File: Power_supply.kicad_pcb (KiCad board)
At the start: 2 copper layers, 160 x 40 mm, 51 parts, among them J1 Transformers, J20 HV_Transformer, J21 LV_Transformer, J22 220V, J23 Transformers, J24 Thyratrone, J25 Anodes_enable, J26 Conn_01x04, J27 Conn_01x04, J28 Conn_01x04, K2 SANYOU_SRD_Form_C, Q10 MPSA42, Q11 STP4NK60ZFP(MJE13003), Q12 2N3904, U4 SG2P

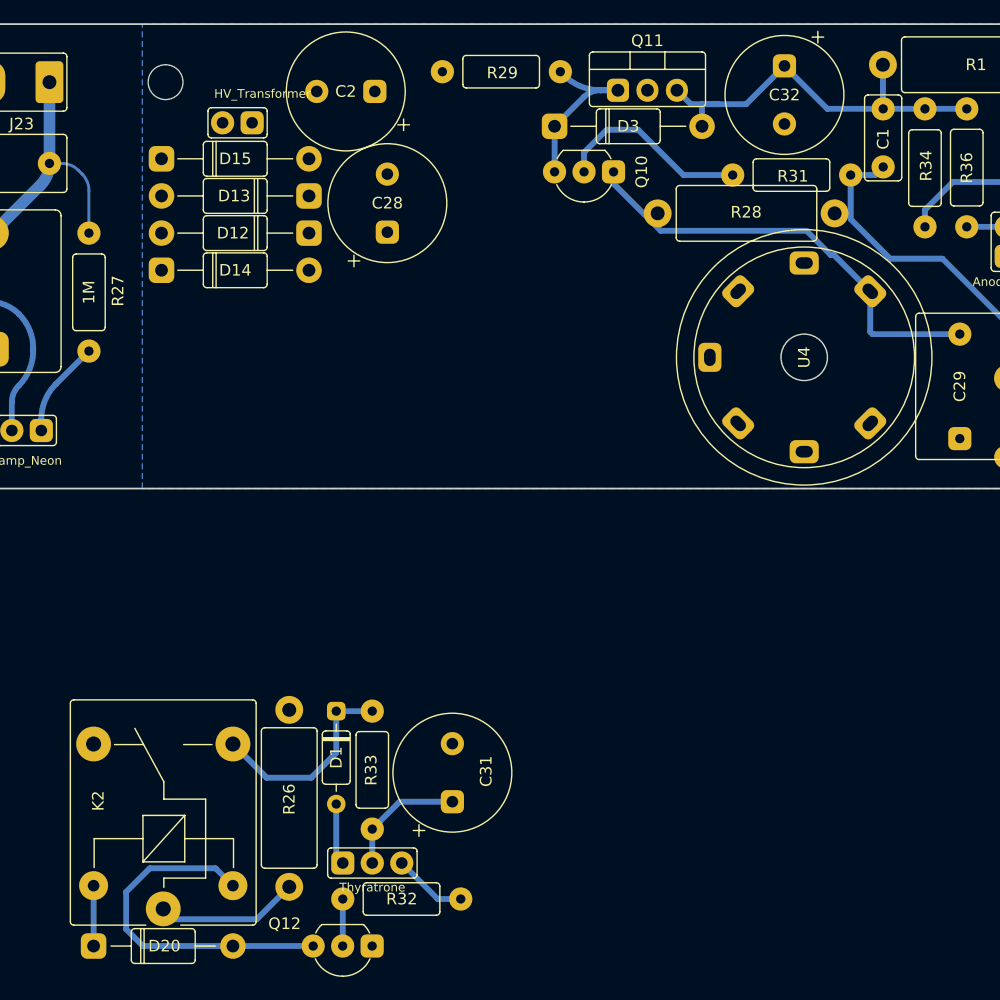
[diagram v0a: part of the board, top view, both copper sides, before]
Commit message: Working on power supply PCB
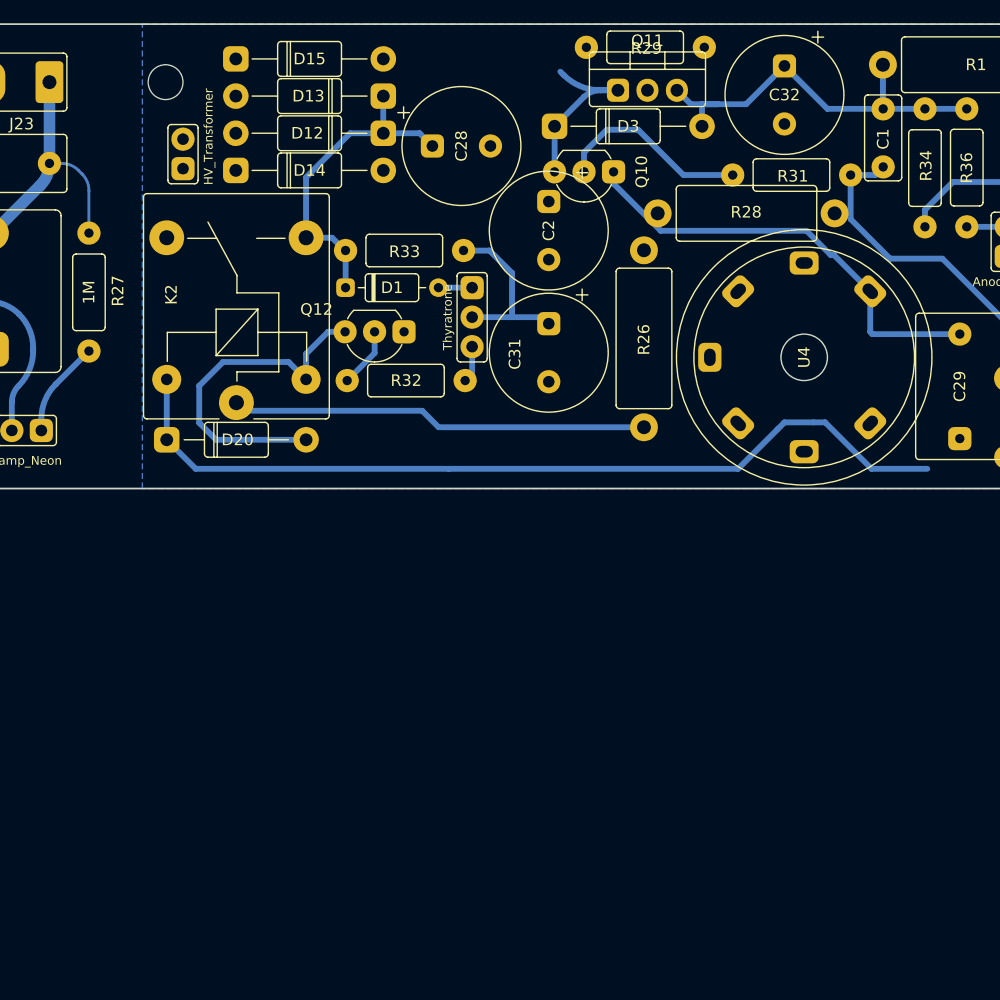
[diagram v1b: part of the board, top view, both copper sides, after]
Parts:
- moved Q12 53.0 mm to (80.0, 116.5)
- moved J24 50.8 mm to (88.4, 112.7), turned to 0 degrees
- moved R33 50.4 mm to (87.7, 109.5), turned to 180 degrees
- moved R26 50.0 mm to (103.2, 124.7)
- moved R32 44.7 mm to (87.8, 120.7)
- moved D20 44.1 mm to (68.1, 125.8)
- moved K2 44.1 mm to (68.1, 122.6)
- moved C31 42.0 mm to (95.0, 115.8), turned to -90 degrees
- moved D1 40.8 mm to (81.5, 112.7), turned to 0 degrees
- moved C2 17.7 mm to (95.0, 105.3), turned to -90 degrees
- moved R29 12.6 mm to (108.4, 92.0)
- moved D15 10.7 mm to (68.0, 93.0)
- moved D13 10.7 mm to (80.8, 96.2)
- moved D12 10.7 mm to (80.8, 99.4)
- moved D14 10.7 mm to (68.0, 102.6)
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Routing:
- net +6V: track 5.20 -> 75.0 mm
- net K1.1: track 12.4 -> 36.0 mm
- net HV: track 17.7 -> 28.3 mm
- net Net-(C31-Pad1): track 10.8 -> 15.6 mm
- net Net-(J24-Pad3): track 6.36 -> 3.17 mm
- net Net-(J24-Pad1): track 5.33 -> 2.90 mm
- net Net-(Q12-Pad2): track 4.05 -> 5.18 mm
- net Net-(D20-Pad2): track 30.6 -> 30.0 mm

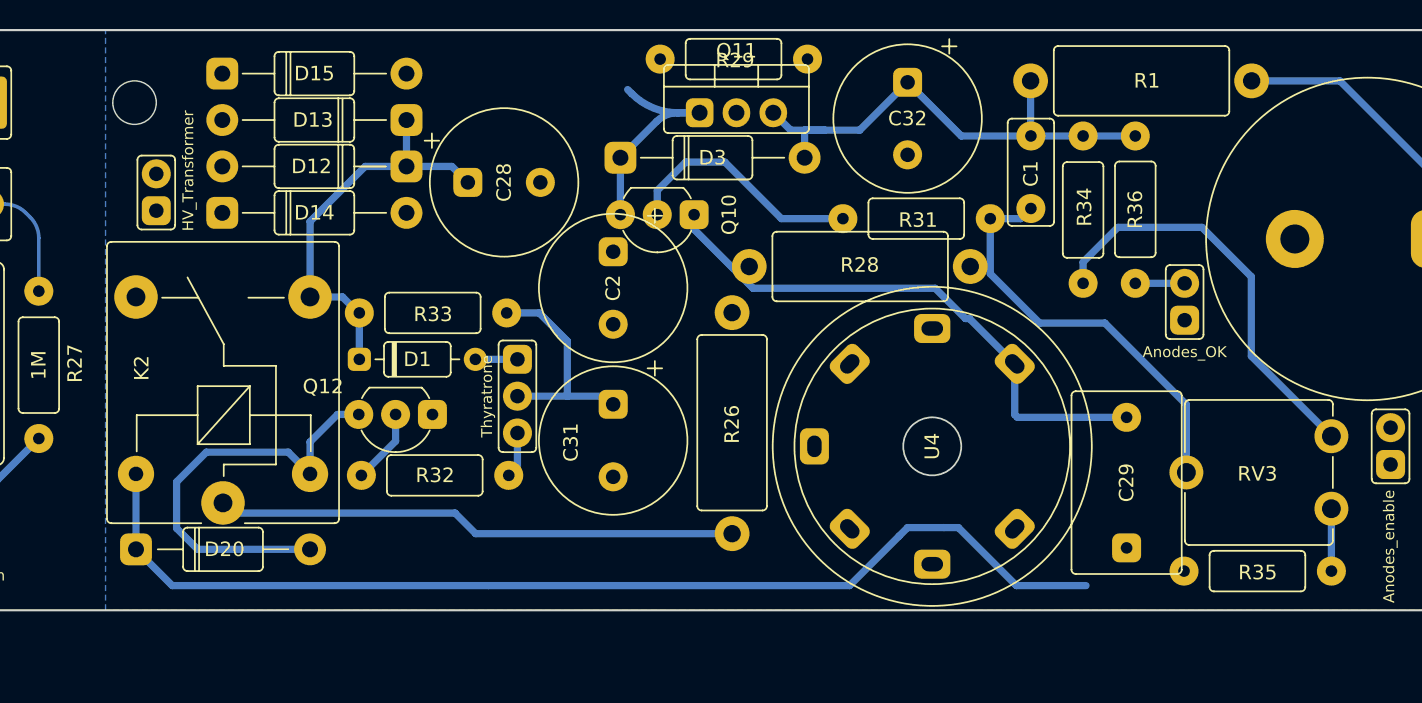
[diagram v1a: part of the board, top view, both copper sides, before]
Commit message: Working on power supply PCB
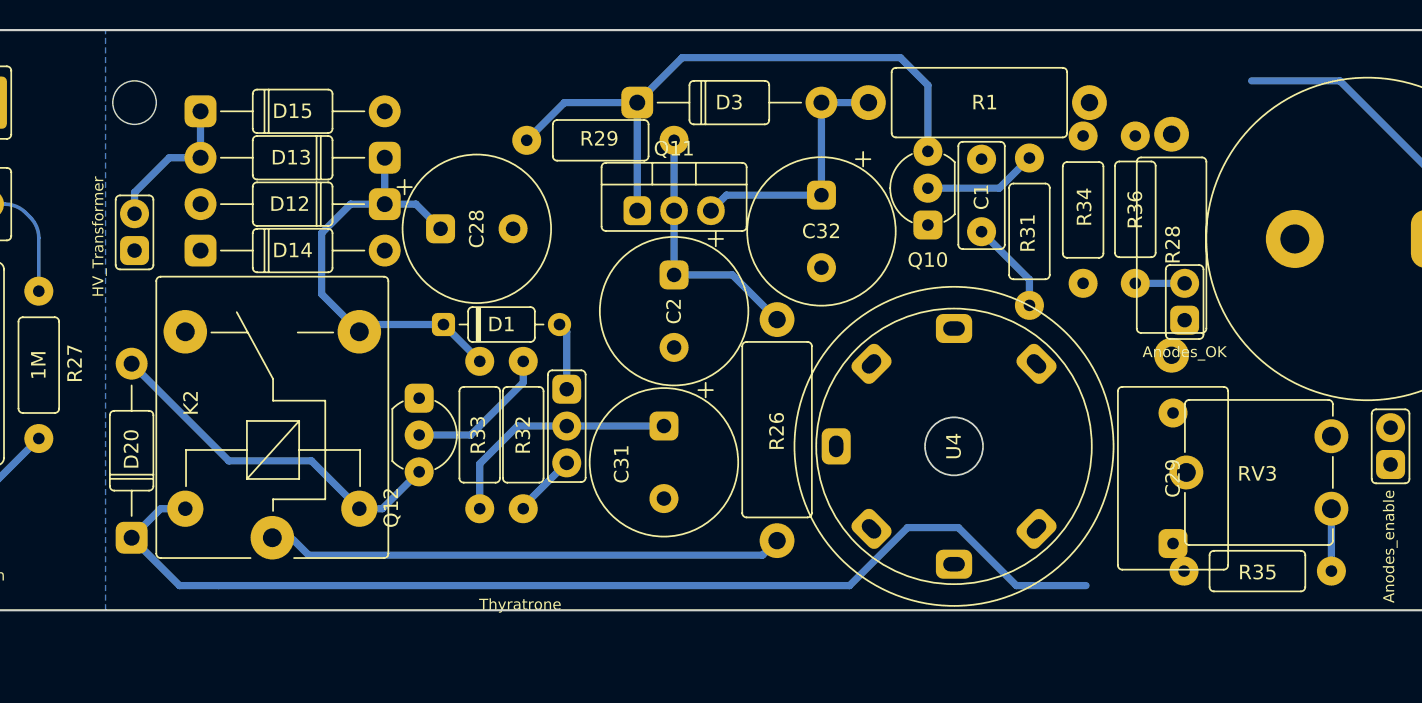
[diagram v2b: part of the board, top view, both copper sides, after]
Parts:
- moved R28 30.5 mm to (133.5, 97.2), turned to -90 degrees
- moved R29 20.2 mm to (89.0, 97.6), turned to 0 degrees
- moved Q10 18.7 mm to (116.7, 100.9), turned to 90 degrees
- moved R33 13.6 mm to (85.8, 123.0), turned to 90 degrees
- moved R1 11.3 mm to (112.6, 95.0)
- moved C32 9.79 mm to (109.4, 101.4)
- moved D20 9.27 mm to (61.8, 119.0), turned to 90 degrees
- moved Q11 8.00 mm to (99.2, 102.5)
- moved R31 6.56 mm to (123.7, 109.0), turned to 90 degrees
- moved D1 6.28 mm to (87.3, 110.3)
- moved C2 4.49 mm to (99.2, 106.9)
- moved K2 4.16 mm to (71.5, 125.0)
- moved J24 3.98 mm to (91.8, 114.8)
- moved D3 3.97 mm to (96.7, 95.0)
- moved C31 3.81 mm to (98.5, 117.3)
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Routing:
- net Net-(Q10-Pad1): track 38.3 -> 0.00 mm
- net Net-(R34-Pad2): track 28.7 -> 0.00 mm
- net Net-(D3-Pad1): track 16.0 -> 42.8 mm
- net Net-(C1-Pad1): track 28.8 -> 6.45 mm
- net Net-(C1-Pad2): track 35.5 -> 17.7 mm
- net Net-(C2-Pad1): track 0.00 -> 17.7 mm
- net Net-(D13-Pad2): track 0.00 -> 10.2 mm
- net Net-(Q10-Pad2): track 16.9 -> 7.86 mm
- net Net-(D20-Pad2): track 30.0 -> 25.0 mm
- net Net-(Q12-Pad2): track 5.18 -> 10.1 mm
- net HV: track 28.3 -> 31.1 mm
- net Net-(J24-Pad1): track 2.90 -> 4.67 mm
- net K1.1: track 36.0 -> 34.3 mm
- net Net-(J24-Pad3): track 3.17 -> 4.43 mm
- net Net-(C31-Pad1): track 15.6 -> 16.9 mm
